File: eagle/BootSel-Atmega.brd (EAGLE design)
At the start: 60.6 x 22.9 mm, 8 parts, among them Q1 20MHz

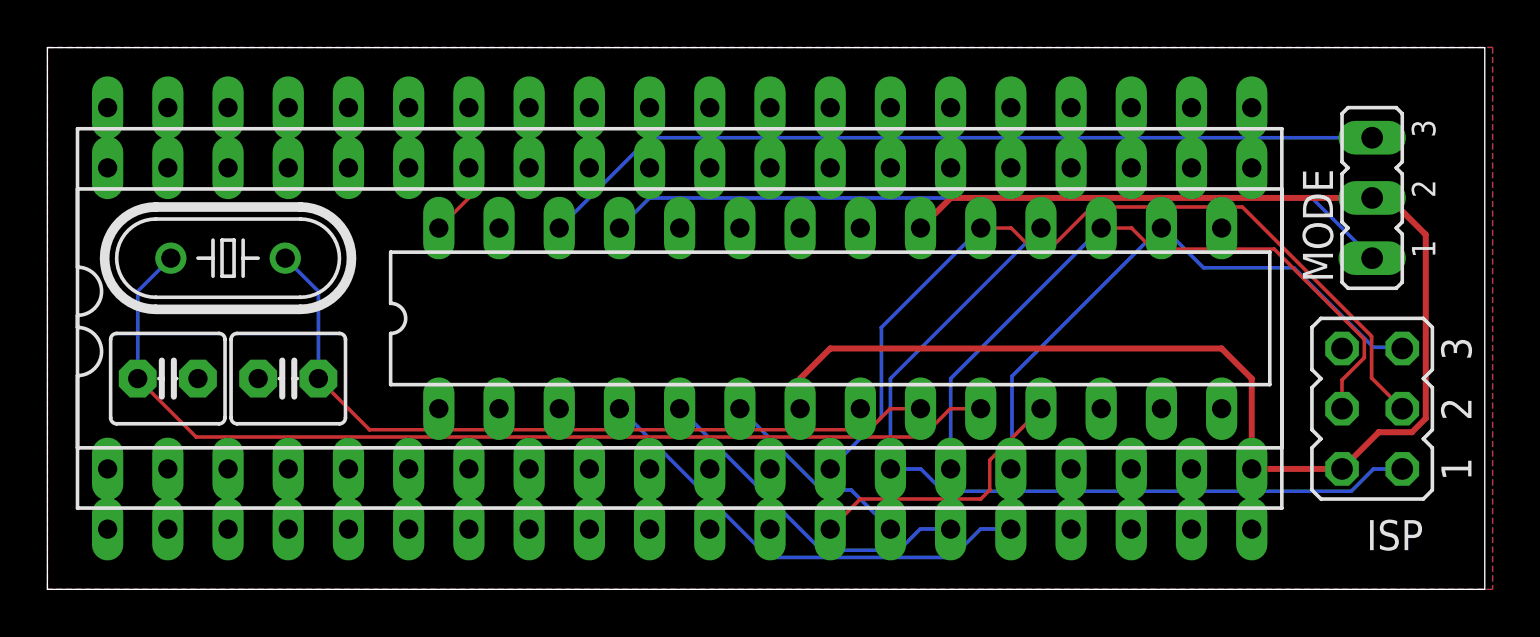
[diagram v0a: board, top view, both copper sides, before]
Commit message: smaller changes
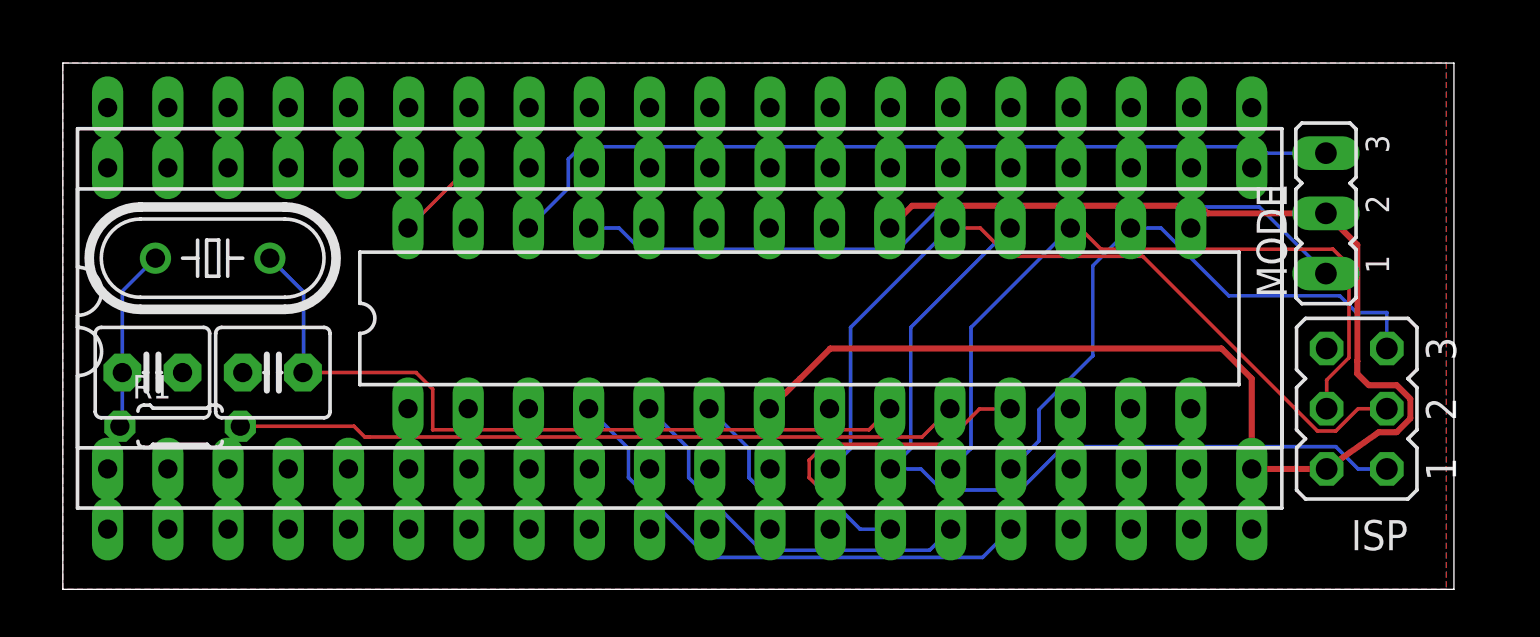
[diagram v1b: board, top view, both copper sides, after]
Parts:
- added R1: 270R, resistor:0204/5
- moved MODE 2.06 mm to (53.9, 15.9)
- moved MEGA 1.30 mm to (31.7, 11.4)
- moved C1 0.70 mm to (9.51, 9.14)
- moved C2 0.70 mm to (4.43, 9.14)
- moved ISP 0.65 mm to (55.2, 7.62)
- moved Q1 0.65 mm to (6.97, 14.0)
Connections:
- net CIA34 renamed /CIA_RESET
- new net N$1: MEGA.10, R1.2
- net N$16: now also R1.1; no longer MEGA.10
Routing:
- net N$16: track 42.7 -> 8.14 mm
- net N$1: track 0.00 -> 30.7 mm
- net /NEWSEL1: track 8.45 -> 10.5 mm
- net /NEWSEL3: track 19.6 -> 21.6 mm
- net /NEWSEL2: track 14.3 -> 16.3 mm
- net MOSI: track 29.2 -> 31.1 mm
- net SCK: track 36.2 -> 34.6 mm
- net ISP_RST: track 25.1 -> 26.1 mm
- net /NEWSEL0: track 11.7 -> 12.7 mm
- net VCC: track 66.2 -> 65.4 mm
- net /CIA_RESET: track 5.61 -> 6.16 mm
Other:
- board size 60.6 x 22.9 mm -> 58.7 x 22.2 mm
- board text added: "AMIGA ATMega Bootselector (c) 2018 Marko Oette retro.oette.info"
